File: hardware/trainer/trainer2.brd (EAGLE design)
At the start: 82.1 x 54.3 mm, 63 parts, among them Q1 2N3906, Q2 2N3906, Q3 2N3906, Q4 2N3906

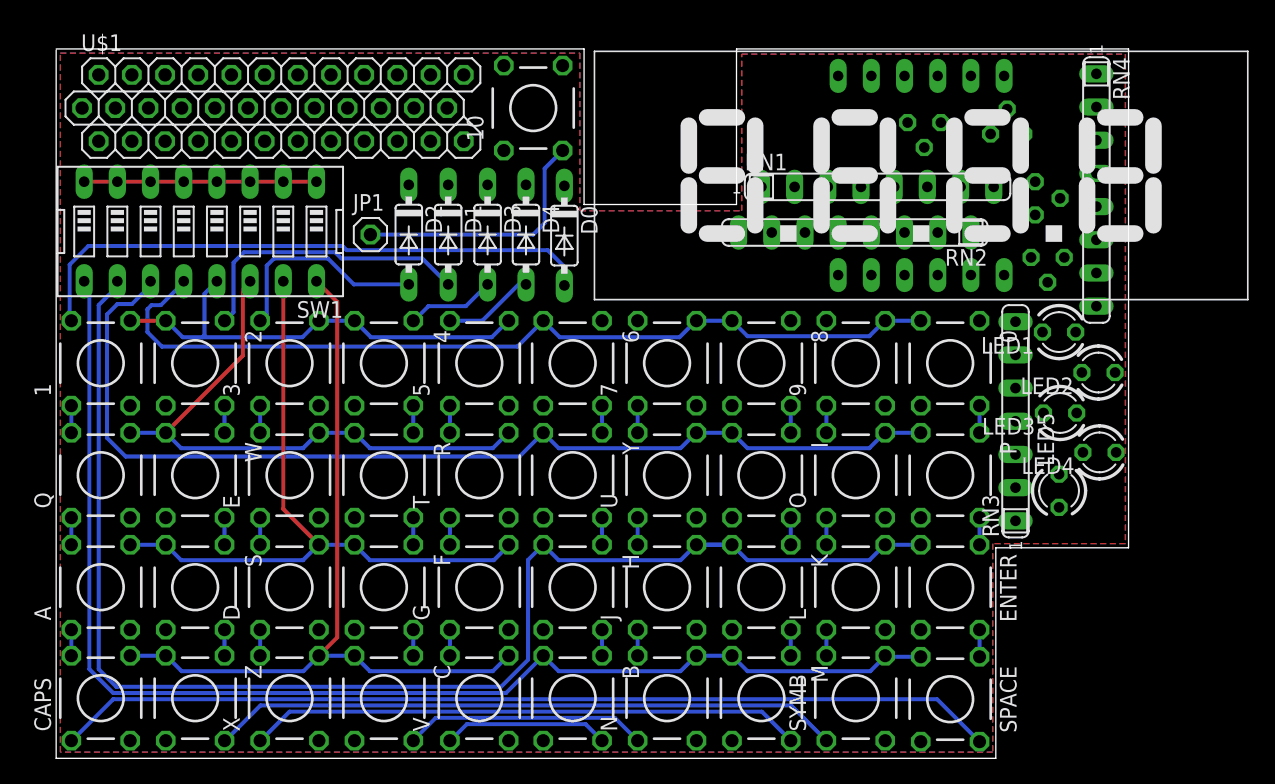
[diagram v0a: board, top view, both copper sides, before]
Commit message: Actualizo trainer2
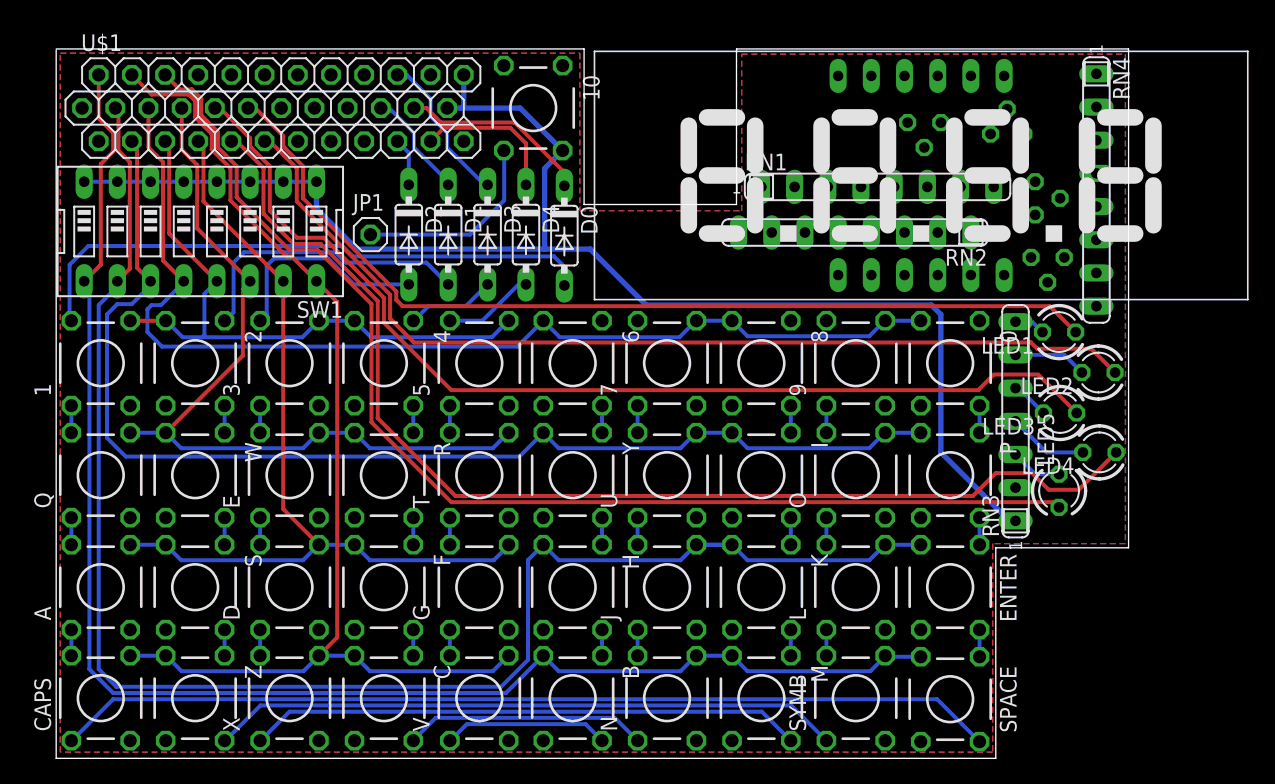
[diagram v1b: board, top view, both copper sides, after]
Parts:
- turned 10 to 270 degrees
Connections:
- removed net LED6: U$1.P24
- removed net N$45: SW1.1, SW1.2, SW1.3, SW1.4, SW1.5, SW1.6, SW1.7, SW1.8
- removed net PUSH1: U$1.P29
- removed net PUSH2: U$1.P20
- removed net PUSH3: U$1.P27
- removed net PUSH4: U$1.P30
- removed net SW1: U$1.P9
- removed net SW2: U$1.P8
- removed net SW3: U$1.P7
- removed net SW4: U$1.P11
- removed net SW5: U$1.P10
- removed net SW6: U$1.P14
- removed net SW7: U$1.P15
- removed net SW8: U$1.P13
- new net COL0: D0.C, U$1.P35
- new net COL1: D1.C, U$1.P32
- new net COL2: D2.C, U$1.P31
- new net COL3: D3.C, U$1.P33
- new net COL4: D4.C, U$1.P34
- net A10: now also U$1.P14
- net A11: now also U$1.P10
- net A12: now also U$1.P11
- net A13: now also U$1.P7
- net A14: now also U$1.P8
- net A15: now also U$1.P6
- net A8: now also U$1.P9
- net A9: now also U$1.P13
- net DIG1: now also U$1.P22; no longer U$1.P19
- net DIG2: now also U$1.P15; no longer U$1.P16
- net DISA: now also U$1.P27; no longer U$1.P25
- net DISC: now also U$1.P25; no longer U$1.P31
- net DISD: now also U$1.P30; no longer U$1.P33
- net DISDP: now also U$1.P26; no longer U$1.P6
- net DISE: now also U$1.P24; no longer U$1.P22
- net DISF: now also U$1.P29; no longer U$1.P17
- net DISG: now also U$1.P21; no longer U$1.P12
- net GND: now also 10.2, SW1.1, SW1.2, SW1.3, SW1.4, SW1.5, SW1.6, SW1.7, SW1.8; no longer 10.1
- net LED1: now also U$1.P20
- net LED2: now also U$1.P19
- net LED3: now also U$1.P17; no longer U$1.P32
- net LED4: now also U$1.P16; no longer U$1.P26
- net LED5: now also U$1.P12; no longer U$1.P21
- net N$15: now also 10.4; no longer 10.3
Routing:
- net GND: track 0.00 -> 110.3 mm
- net LED5: track 0.00 -> 90.3 mm
- net LED4: track 0.00 -> 88.7 mm
- net LED3: track 0.00 -> 80.1 mm
- net LED2: track 0.00 -> 75.0 mm
- net LED1: track 0.00 -> 72.7 mm
- net A8: track 60.8 -> 84.4 mm
- net N$45: track 17.8 -> 0.00 mm
- net A15: track 97.4 -> 114.6 mm
- net A10: track 45.2 -> 60.6 mm
- net COL0: track 0.00 -> 14.6 mm
- net A12: track 68.0 -> 82.3 mm
- net A14: track 107.4 -> 121.5 mm
- net A9: track 52.3 -> 65.7 mm
- net A11: track 35.8 -> 48.2 mm
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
